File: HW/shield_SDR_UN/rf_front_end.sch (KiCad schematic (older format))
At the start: 47 parts, among them Q1 MOSFET_P, U1 MAX5864, U2 MAX2830

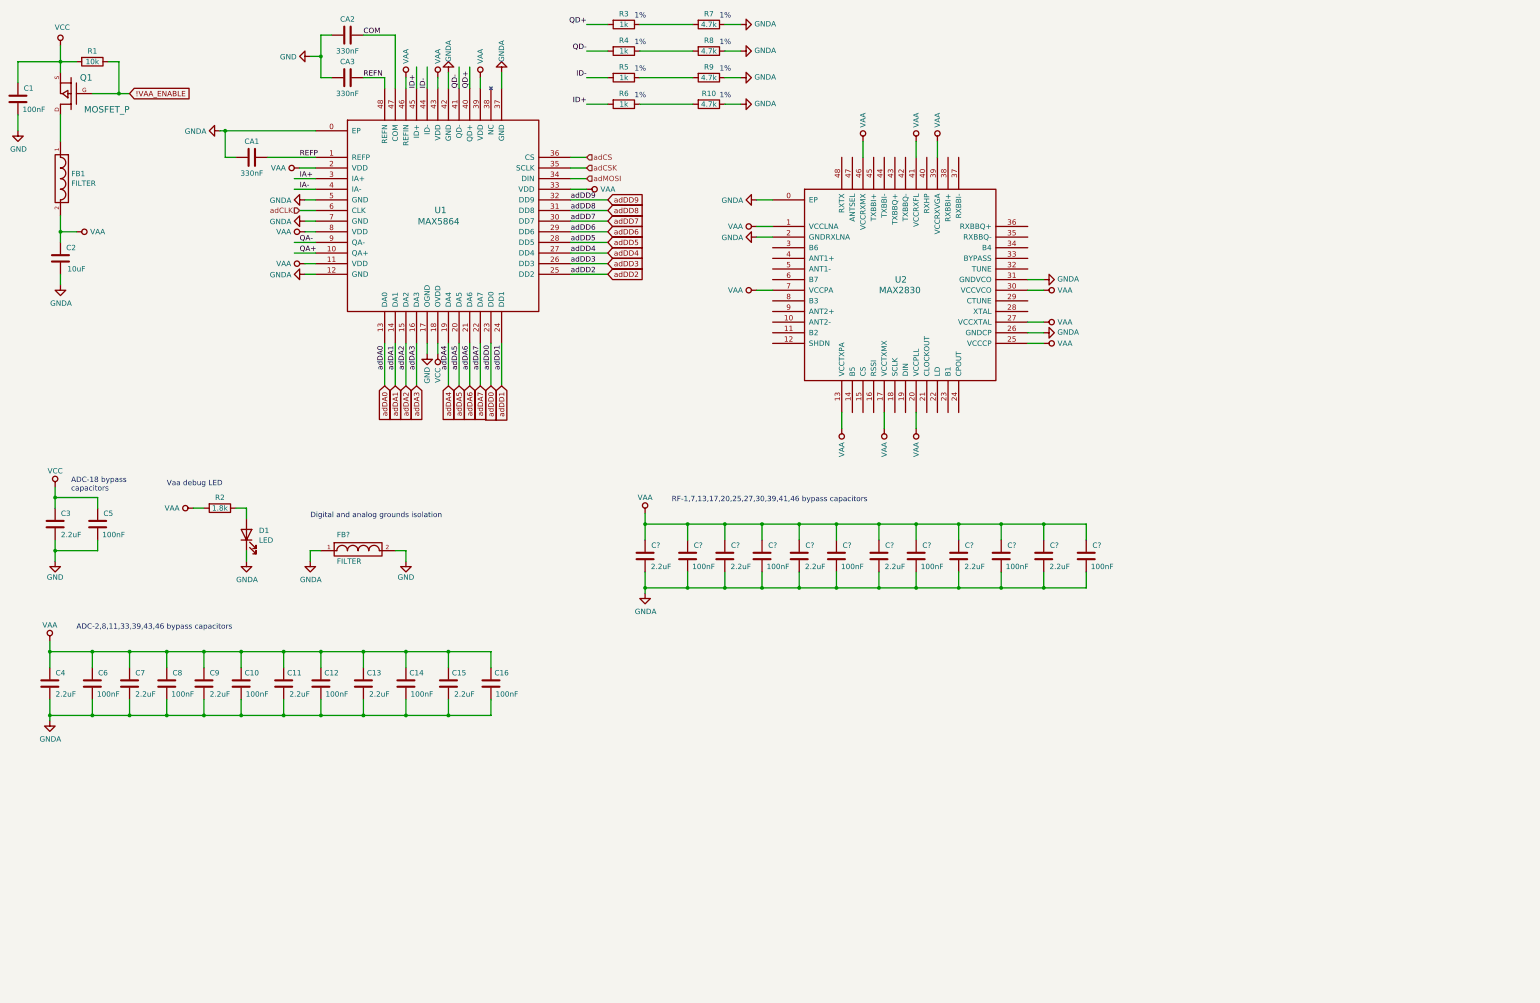
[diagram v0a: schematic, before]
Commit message: RF-Frontend balun
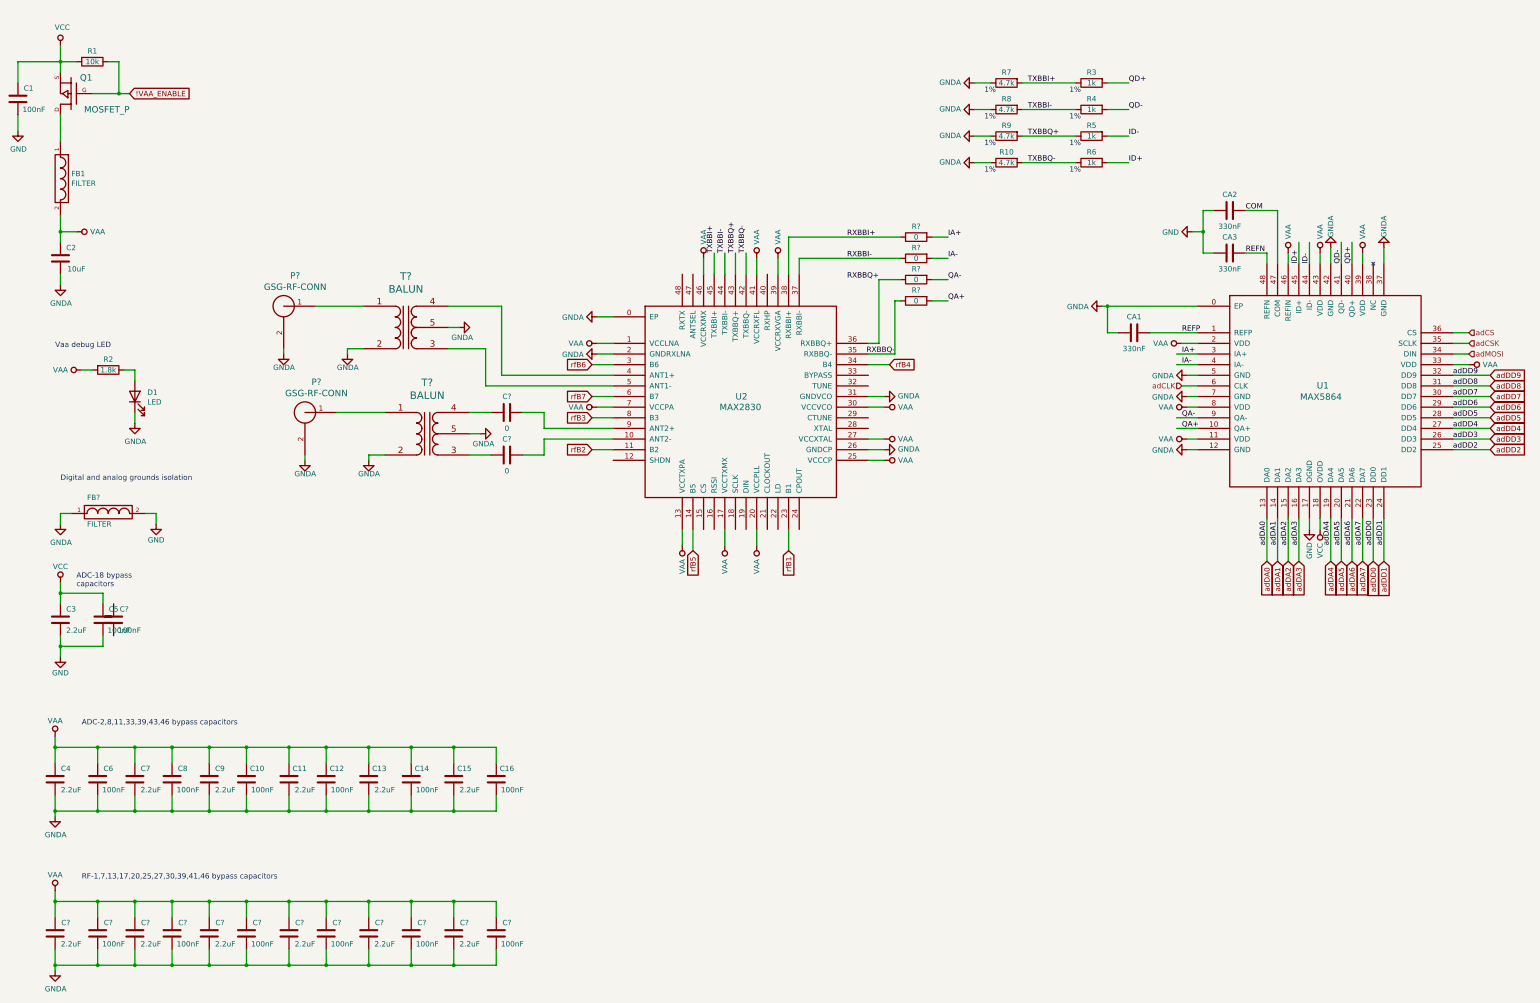
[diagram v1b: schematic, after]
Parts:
- added C?: 100nF, symbol Device:C
- added C? (x2): 0, symbol Device:C
- added P? (x2): GSG-RF-CONN, symbol hackrf-one-rescue:GSG-RF-CONN
- added R? (x4): 0, symbol Device:R
- added T? (x2): BALUN, symbol hackrf-one-rescue:BALUN
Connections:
- net labels added: RXBBI+, RXBBI-, RXBBQ+, RXBBQ-, TXBBI+, TXBBI-, TXBBQ+, TXBBQ-, rfB1, rfB2, rfB3, rfB4, rfB5, rfB6, rfB7
- wire segments 212 -> 261
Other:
- moved on the sheet: C10, C11, C12, C13, C14, C15, C16, C3, C4, C5, C6, C7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
